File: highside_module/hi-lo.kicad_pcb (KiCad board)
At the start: 2 copper layers, 43.4 x 15.5 mm, 30 parts, among them M601 CONN_1, P601 CONN_3X2, P602 CONN_2, P603 CONN_6, P604 CONN_2, U601 TC4427, U602 TC4427, U603 TC4427

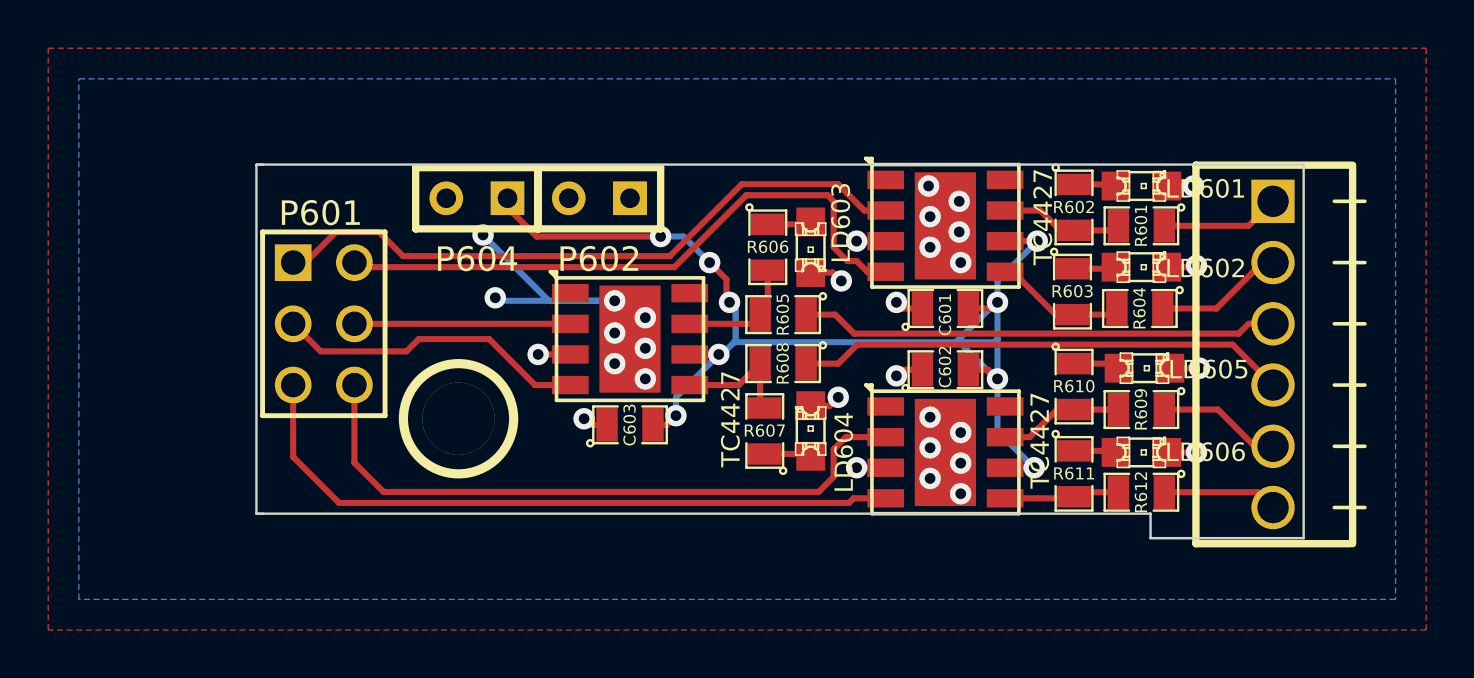
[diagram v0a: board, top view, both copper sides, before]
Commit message: sorry for party
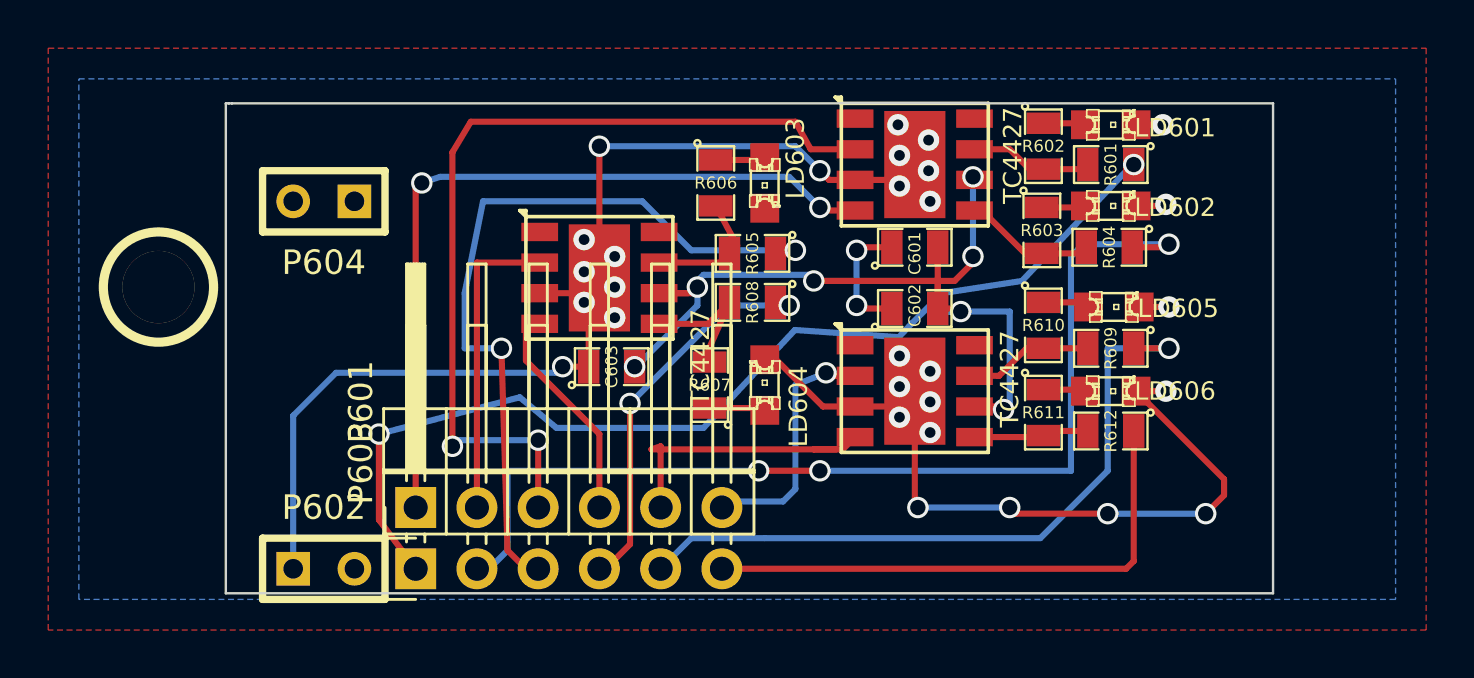
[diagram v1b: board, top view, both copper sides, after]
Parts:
- P601: footprint pin_array_3x2 -> Pin_Headers:Pin_Header_Angled_1x06_Pitch2.54mm
- P603: footprint OSTVN06A150 -> Pin_Headers:Pin_Header_Angled_1x06_Pitch2.54mm
- moved P603 36.7 mm to (182.9, 167.6), turned to 90 degrees
- moved P602 19.2 mm to (179.1, 167.6), turned to 0 degrees
- moved M601 13.6 mm to (172.2, 156.0)
- moved G601 9.66 mm to (214.9, 164.6)
- moved P601 8.52 mm to (182.9, 165.1), turned to 90 degrees
- moved P604 6.35 mm to (179.1, 152.4)
- moved R606 3.43 mm to (195.3, 151.6)
- moved LD603 3.28 mm to (197.4, 151.6)
- moved R607 2.98 mm to (195.1, 160.0)
- moved LD602 2.84 mm to (211.7, 152.6)
- moved U602 2.84 mm to (190.5, 155.6)
- moved C601 2.84 mm to (203.6, 154.3)
- moved C602 2.84 mm to (203.6, 156.8)
- moved LD601 2.84 mm to (211.7, 149.2)
- moved LD606 2.84 mm to (211.7, 160.3)
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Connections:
- P601 pad 1: /H_IN3 -> /H_IN1
- P601 pad 2: /H_IN1 -> /H_IN2
- P601 pad 3: /H_IN4 -> /H_IN3
- P601 pad 4: /H_IN2 -> /H_IN4
- P602 pad 2: (no net) -> 5V
- P604 pad 2: (no net) -> 12V
- U601 pad 1: (no net) -> Net-(U601-Pad1)
- U601 pad 8: (no net) -> Net-(U601-Pad8)
- U602 pad 1: (no net) -> Net-(U602-Pad1)
- U602 pad 8: (no net) -> Net-(U602-Pad8)
- U603 pad 1: (no net) -> Net-(U603-Pad1)
- U603 pad 8: (no net) -> Net-(U603-Pad8)
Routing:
- net GND: track 71.8 -> 132.2 mm, vias 32 -> 31
- net /HL1: track 4.93 -> 43.2 mm, vias 0 -> 2
- net /HL2: track 5.36 -> 43.0 mm, vias 0 -> 3
- net /HL5: track 5.14 -> 29.3 mm, vias 0 -> 1
- net /HL6: track 4.77 -> 22.6 mm
- net /H_IN6: track 27.4 -> 10.3 mm, vias 0 -> 1
- net /H_IN5: track 28.4 -> 12.6 mm
- net /HL3: track 19.9 -> 32.3 mm, vias 0 -> 2
- net /H_IN3: track 27.2 -> 36.7 mm, vias 0 -> 2
- net /VP: track 51.6 -> 42.1 mm, vias 9 -> 7
- net /H_IN1: track 25.8 -> 32.2 mm, vias 0 -> 3
- net /HL4: track 20.4 -> 16.4 mm, vias 0 -> 2
- net /H_IN2: track 8.95 -> 12.8 mm
- net /H_IN4: track 13.0 -> 9.31 mm
- net Net-(R607-Pad2): track 5.21 -> 6.06 mm
- added copper zone on B.Cu, net /VP
- removed copper zone on B.Cu, net GND
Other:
- board size 43.4 x 15.5 mm -> 43.4 x 20.3 mm
- board text added: "R.03 rusefi.com"
- board text removed: "GND"
- board text removed: "HI-LO1"
- board text removed: "HI-LO2"
- board text removed: "HI-LO3"
- board text removed: "HI-LO4"
- board text removed: "HI-LO5"
- board text removed: "HI-LO6"
- board text removed: "R.02 https://code.google.com/p/daecu/"
- board text removed: "VP"
- board text removed: "for RUSEFI.com"
